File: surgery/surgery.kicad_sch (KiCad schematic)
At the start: 9 parts, among them J1 Conn_01x05_Pin, Q1 bc337, U2 LM66100Q, U3 LM66100Q, U4 LM66100Q

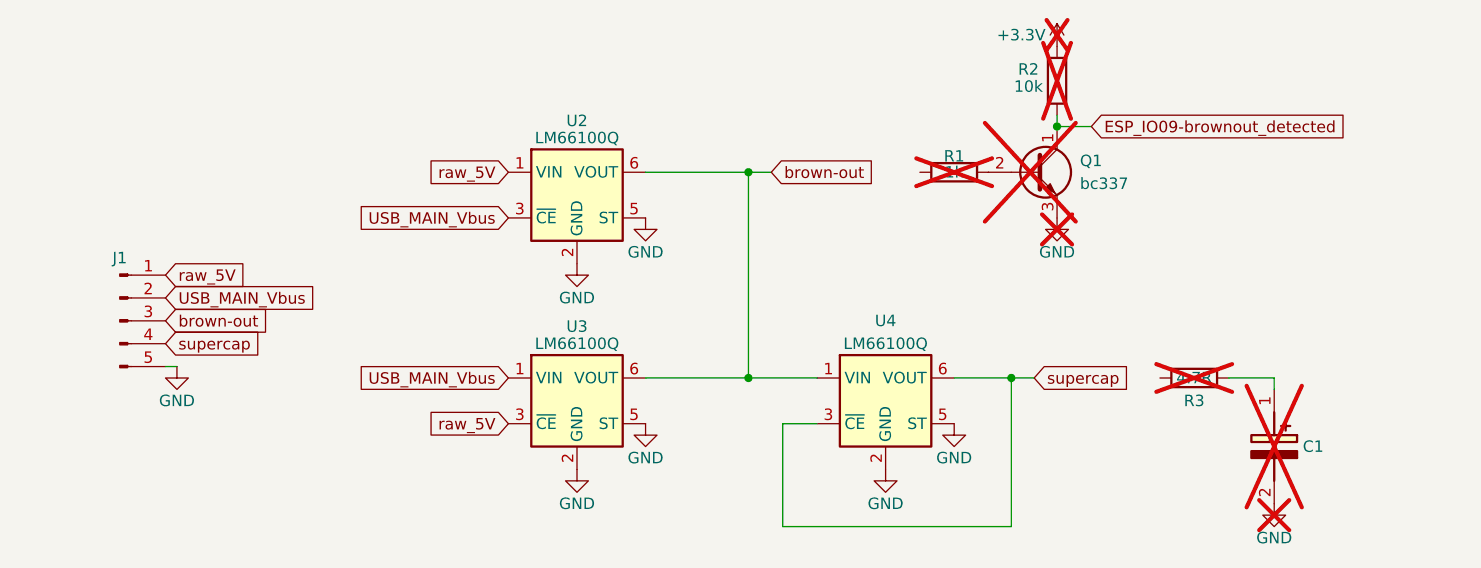
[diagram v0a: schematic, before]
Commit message: plotting
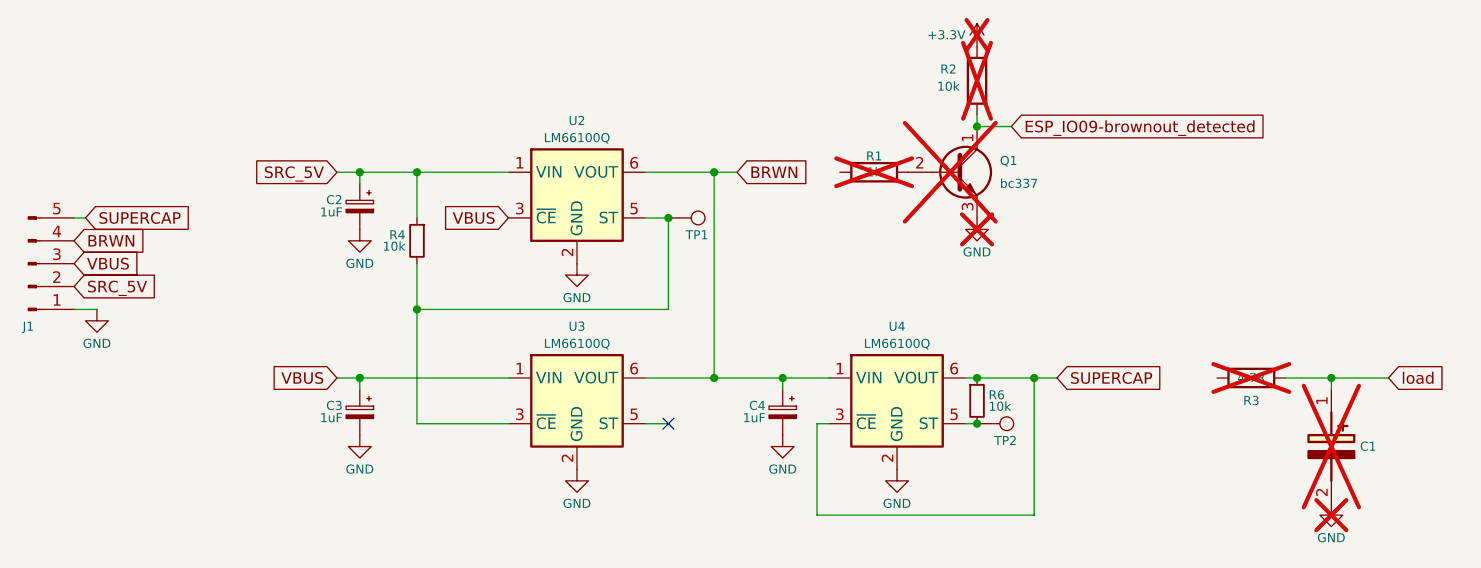
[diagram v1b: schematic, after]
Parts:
- added C2, C3, C4: 1uF, Capacitor_Tantalum_SMD:CP_EIA-3216-18_Kemet-A, symbol Device:C_Polarized_Small
- added R4, R6: 10k, Resistor_SMD:R_0805_2012Metric, symbol Device:R_Small
- added TP1, TP2: TestPoint, TestPoint:TestPoint_Loop_D1.80mm_Drill1.0mm_Beaded, symbol Connector:TestPoint
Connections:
- net GND: now also J1.1 (Pin_1), C2.2, C3.2, C4.2; no longer J1.5 (Pin_5), U2.5 (ST), U3.5 (ST), U4.5 (ST)
- net load: now reaches C1.1 (+), R3.1
- net USB_MAIN_Vbus renamed VBUS
- net VBUS: now also J1.3 (Pin_3), C3.1; no longer J1.2 (Pin_2)
- net brown-out renamed BRWN
- net BRWN: now also J1.4 (Pin_4), C4.1; no longer J1.3 (Pin_3)
- removed net raw_5V: J1.1 (Pin_1), U2.1 (VIN), U3.3 (~{CE})
- net supercap renamed SUPERCAP
- net SUPERCAP: now also J1.5 (Pin_5), R6.1; no longer J1.4 (Pin_4)
- new net: R4.2, TP1.1, U2.5 (ST), U3.3 (~{CE})
- new net: R6.2, TP2.1, U4.5 (ST)
- new net SRC_5V: C2.1, J1.2 (Pin_2), R4.1, U2.1 (VIN)
- no-connect marks 0 -> 1
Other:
- moved on the sheet: C1, J1, Q1, R1, R2, R3, U4
